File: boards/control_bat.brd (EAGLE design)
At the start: 101.6 x 30.5 mm, 18 parts, among them U1 579-MCP1703T-3002ECB, U2 771-LPC824M201JDH20J, U3 888-XB24CZ7PIS-004

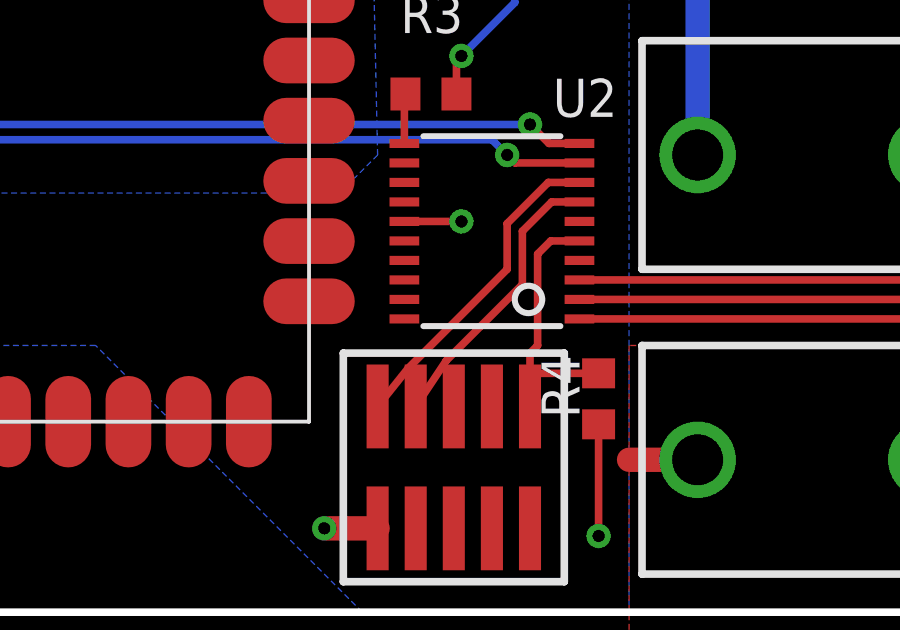
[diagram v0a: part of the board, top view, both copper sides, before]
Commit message: Fix overlap
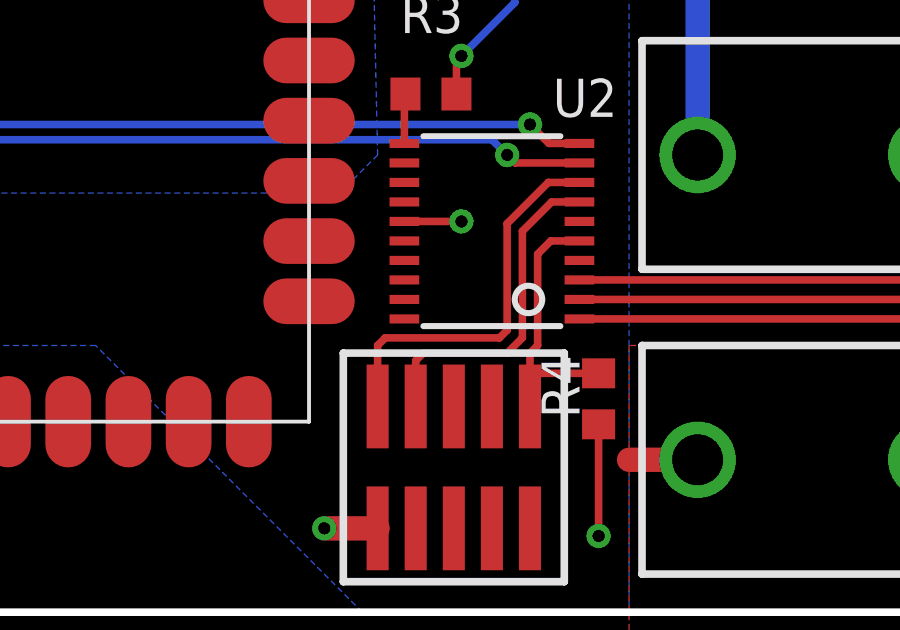
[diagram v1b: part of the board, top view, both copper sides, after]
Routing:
- net SWDIO: track 10.8 -> 13.1 mm
- net SWCLK: track 9.51 -> 11.3 mm
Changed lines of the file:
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@@
 <signal name="SWDIO">
 <contactref element="JP3" pad="2"/>
-<wire x1="36.068" y1="6.858" x2="37.084" y2="8.128" width="0.254" layer="1"/>
-<wire x1="37.084" y1="8.128" x2="40.386" y2="11.43" width="0.254" layer="1"/>
-<wire x1="40.386" y1="11.43" x2="40.386" y2="12.954" width="0.254" layer="1"/>
 <wire x1="40.386" y1="12.954" x2="41.757" y2="14.325" width="0.254" layer="1"/>
 <contactref element="U2" pad="8"/>
 <wire x1="41.757" y1="14.325" x2="42.7958" y2="14.325" width="0.254" layer="1"/>
+<wire x1="36.068" y1="6.858" x2="36.068" y2="8.89" width="0.254" layer="1"/>
+<wire x1="36.068" y1="8.89" x2="36.322" y2="9.144" width="0.254" layer="1"/>
+<wire x1="36.322" y1="9.144" x2="40.132" y2="9.144" width="0.254" layer="1"/>
+<wire x1="40.132" y1="9.144" x2="40.386" y2="9.398" width="0.254" layer="1"/>
+<wire x1="40.386" y1="9.398" x2="40.386" y2="12.954" width="0.254" layer="1"/>
 </signal>
 <signal name="SWCLK">
 <contactref element="JP3" pad="4"/>
-<wire x1="37.338" y1="6.858" x2="38.354" y2="8.382" width="0.254" layer="1"/>
-<wire x1="38.354" y1="8.382" x2="40.894" y2="10.922" width="0.254" layer="1"/>
-<wire x1="40.894" y1="10.922" x2="40.894" y2="12.7" width="0.254" layer="1"/>
 <wire x1="40.894" y1="12.7" x2="41.869" y2="13.675" width="0.254" layer="1"/>
 <contactref element="U2" pad="7"/>
 <wire x1="41.869" y1="13.675" x2="42.7958" y2="13.675" width="0.254" layer="1"/>
+<wire x1="37.338" y1="6.858" x2="37.338" y2="8.382" width="0.254" layer="1"/>
+<wire x1="37.338" y1="8.382" x2="37.592" y2="8.636" width="0.254" layer="1"/>
+<wire x1="37.592" y1="8.636" x2="40.386" y2="8.636" width="0.254" layer="1"/>
+<wire x1="40.386" y1="8.636" x2="40.894" y2="9.144" width="0.254" layer="1"/>
+<wire x1="40.894" y1="9.144" x2="40.894" y2="12.7" width="0.254" layer="1"/>
 </signal>
 <signal name="RST">
@@
 </signal>
 </signals>
+<errors>
+</errors>
 </board>
 </drawing>
